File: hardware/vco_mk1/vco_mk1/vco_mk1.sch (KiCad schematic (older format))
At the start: 86 parts, among them J1 power supply, J2 control in, J3 signal out, J4 Conn_01x03_Male, J5 BCM847 breakout socket, J6 Conn_01x01_Male, Q1 BCM847, Q2 BC547, Q3 BC547, Q4 2N7000, Q5 BC547, Q6 BC327, U1 LM324, U2 LM324, U3 74HC86

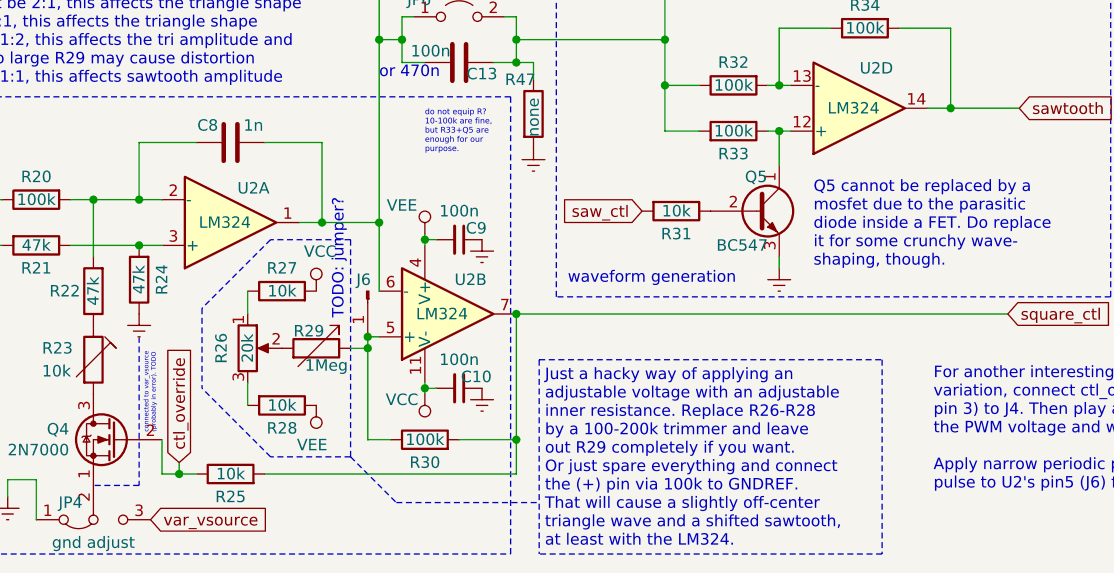
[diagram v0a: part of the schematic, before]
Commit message: triangle center adjust: add 0-Ohm-resistor to GNDREF
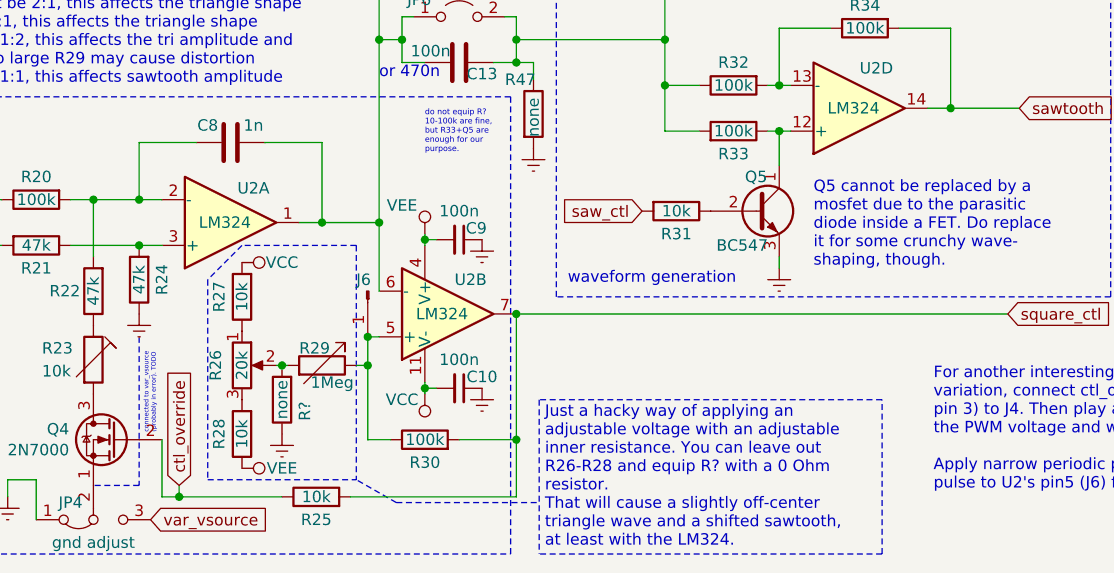
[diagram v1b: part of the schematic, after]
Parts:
- added R?: none, Resistor_SMD:R_0805_2012Metric_Pad1.15x1.40mm_HandSolder, symbol Device:R
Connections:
- net GNDREF: now also R?.1
- net at R26.2, R29.2: now also R?.2
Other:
- note added: "Just a hacky way of applying an\nadjustable voltage with an adjustable\ninner resistance. You can leave out\nR26-R28 and equip R? with a 0 Ohm\nresistor.\nThat will cause a slightly off-center\ntriangle wave and a shifted sawtooth,\nat least with the LM324."
- note removed: "Just a hacky way of applying an\nadjustable voltage with an adjustable\ninner resistance. Replace R26-R28\nby a 100-200k trimmer and leave\nout R29 completely if you want.\nOr just spare everything and connect\nthe (+) pin via 100k to GNDREF.\nThat will cause a slightly off-center\ntriangle wave and a shifted sawtooth,\nat least with the LM324."
- note removed: "TODO: jumper?"
- moved on the sheet: R25, R26, R27, R28, R29
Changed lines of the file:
@@
 $EndComp
 Wire Wire Line
-	2375 7400 3475 7400
-Wire Wire Line
-	3475 7400 3475 7250
+	2750 7500 3475 7500
+Wire Wire Line
+	3475 7500 3475 7250
 Wire Wire Line
 	3475 7250 3475 6700
@@
 Wire Wire Line
 	2875 6800 2825 6800
-Wire Wire Line
-	2825 6800 2825 6850
 $Comp
 L power:VCC #PWR026
@@
 U 1 1 5D5CE3BE
 P 3225 7025
-F 0 "C10" V 3175 7100 50  0000 C CNN
+F 0 "C10" V 3175 7125 50  0000 C CNN
 F 1 "100n" V 3100 7025 50  0000 C CNN
 F 2 "Capacitor_SMD:C_0805_2012Metric_Pad1.15x1.40mm_HandSolder" H 3225 7025 50  0001 C CNN
@@
 L Device:R R27
 U 1 1 5D9107CB
-P 2450 6600
-F 0 "R27" V 2550 6600 50  0000 C CNN
-F 1 "10k" V 2450 6600 50  0000 C CNN
-F 2 "Resistor_SMD:R_0805_2012Metric_Pad1.15x1.40mm_HandSolder" V 2380 6600 50  0001 C CNN
-F 3 "~" H 2450 6600 50  0001 C CNN
-	1    2450 6600
-	0    -1   -1   0
+P 2275 6625
+F 0 "R27" V 2375 6625 50  0000 C CNN
+F 1 "10k" V 2275 6625 50  0000 C CNN
+F 2 "Resistor_SMD:R_0805_2012Metric_Pad1.15x1.40mm_HandSolder" V 2205 6625 50  0001 C CNN
+F 3 "~" H 2275 6625 50  0001 C CNN
+	1    2275 6625
+	-1   0    0    1
 $EndComp
 $Comp
 L Device:R R28
 U 1 1 5D910D8F
-P 2450 7100
-F 0 "R28" V 2550 7100 50  0000 C CNN
-F 1 "10k" V 2450 7100 50  0000 C CNN
-F 2 "Resistor_SMD:R_0805_2012Metric_Pad1.15x1.40mm_HandSolder" V 2380 7100 50  0001 C CNN
-F 3 "~" H 2450 7100 50  0001 C CNN
-	1    2450 7100
-	0    1    1    0
+P 2275 7225
+F 0 "R28" V 2375 7225 50  0000 C CNN
+F 1 "10k" V 2275 7225 50  0000 C CNN
+F 2 "Resistor_SMD:R_0805_2012Metric_Pad1.15x1.40mm_HandSolder" V 2205 7225 50  0001 C CNN
+F 3 "~" H 2275 7225 50  0001 C CNN
+	1    2275 7225
+	-1   0    0    1
 $EndComp
 $Comp
 L Device:R_POT R26
 U 1 1 5D911866
-P 2300 6850
-F 0 "R26" V 2185 6850 50  0000 C CNN
-F 1 "20k" V 2300 6850 50  0000 C CNN
-F 2 "Potentiometer_THT:Potentiometer_Runtron_RM-065_Vertical" H 2300 6850 50  0001 C CNN
-F 3 "~" H 2300 6850 50  0001 C CNN
-	1    2300 6850
+P 2275 6925
+F 0 "R26" V 2160 6925 50  0000 C CNN
+F 1 "20k" V 2275 6925 50  0000 C CNN
+F 2 "Potentiometer_THT:Potentiometer_Runtron_RM-065_Vertical" H 2275 6925 50  0001 C CNN
+F 3 "~" H 2275 6925 50  0001 C CNN
+	1    2275 6925
 	1    0    0    -1
 $EndComp
@@
 L power:VEE #PWR024
 U 1 1 5D92BF20
-P 2600 7100
-F 0 "#PWR024" H 2600 6950 50  0001 C CNN
-F 1 "VEE" H 2618 7273 50  0000 C CNN
-F 2 "" H 2600 7100 50  0001 C CNN
-F 3 "" H 2600 7100 50  0001 C CNN
-	1    2600 7100
-	-1   0    0    1
+P 2275 7375
+F 0 "#PWR024" H 2275 7225 50  0001 C CNN
+F 1 "VEE" V 2275 7550 50  0000 C CNN
+F 2 "" H 2275 7375 50  0001 C CNN
+F 3 "" H 2275 7375 50  0001 C CNN
+	1    2275 7375
+	0    1    1    0
 $EndComp
 $Comp
 L power:VCC #PWR023
 U 1 1 5D931D60
-P 2600 6600
-F 0 "#PWR023" H 2600 6450 50  0001 C CNN
-F 1 "VCC" H 2617 6773 50  0000 C CNN
-F 2 "" H 2600 6600 50  0001 C CNN
-F 3 "" H 2600 6600 50  0001 C CNN
-	1    2600 6600
-	1    0    0    -1
+P 2275 6475
+F 0 "#PWR023" H 2275 6325 50  0001 C CNN
+F 1 "VCC" V 2275 6650 50  0000 C CNN
+F 2 "" H 2275 6475 50  0001 C CNN
+F 3 "" H 2275 6475 50  0001 C CNN
+	1    2275 6475
+	0    1    1    0
 $EndComp
 $Comp
 L Device:R_Variable R29
 U 1 1 5D95EF15
-P 2600 6850
-F 0 "R29" V 2675 6750 50  0000 L CNN
-F 1 "1Meg" V 2525 6800 50  0000 L CNN
-F 2 "Potentiometer_THT:Potentiometer_Runtron_RM-065_Vertical" V 2530 6850 50  0001 C CNN
-F 3 "~" H 2600 6850 50  0001 C CNN
-	1    2600 6850
+P 2625 6925
+F 0 "R29" V 2700 6825 50  0000 L CNN
+F 1 "1Meg" V 2550 6875 50  0000 L CNN
+F 2 "Potentiometer_THT:Potentiometer_Runtron_RM-065_Vertical" V 2555 6925 50  0001 C CNN
+F 3 "~" H 2625 6925 50  0001 C CNN
+	1    2625 6925
 	0    1    -1   0
 $EndComp
@@
 $EndComp
 Wire Wire Line
-	2000 7400 2075 7400
-Wire Wire Line
-	2000 7350 2000 7400
-Text GLabel 2000 7350 1    50   Input ~ 0
+	2000 7500 2450 7500
+Wire Wire Line
+	2000 7450 2000 7500
+Text GLabel 2000 7450 1    50   Input ~ 0
 ctl_override
-Connection ~ 2000 7400
-Wire Wire Line
-	1925 7400 2000 7400
-Wire Wire Line
-	1925 7250 1925 7400
 $Comp
 L Transistor_FET:2N7000 Q4
@@
 L Device:R R25
 U 1 1 5CF3A8E6
-P 2225 7400
-F 0 "R25" V 2125 7400 50  0000 C CNN
-F 1 "10k" V 2225 7400 50  0000 C CNN
-F 2 "Resistor_SMD:R_0805_2012Metric_Pad1.15x1.40mm_HandSolder" V 2155 7400 50  0001 C CNN
-F 3 "~" H 2225 7400 50  0001 C CNN
-	1    2225 7400
+P 2600 7500
+F 0 "R25" V 2500 7500 50  0000 C CNN
+F 1 "10k" V 2600 7500 50  0000 C CNN
+F 2 "Resistor_SMD:R_0805_2012Metric_Pad1.15x1.40mm_HandSolder" V 2530 7500 50  0001 C CNN
+F 3 "~" H 2600 7500 50  0001 C CNN
+	1    2600 7500
 	0    -1   -1   0
 $EndComp
@@
 	1    0    0    -1
 $EndComp
-Wire Wire Line
-	2300 6600 2300 6700
-Wire Wire Line
-	2300 7100 2300 7000
-Wire Wire Line
-	2750 6850 2825 6850
-Connection ~ 2825 6850
-Wire Wire Line
-	2825 6850 2825 7250
-Wire Notes Line
-	2750 6375 2400 6375
-Wire Notes Line
-	2750 7325 2400 7325
-Wire Notes Line
-	2750 6375 2750 7325
-Wire Notes Line
-	2400 7325 2100 7025
-Wire Notes Line
-	2400 6375 2100 6675
-Wire Notes Line
-	2100 6675 2100 7025
-Wire Notes Line
-	2750 7325 2950 7525
 Text Notes 3600 7725 0    50   ~ 0
-Just a hacky way of applying an\nadjustable voltage with an adjustable\ninner resistance. Replace R26-R28\nby a 100-200k trimmer and leave\nout R29 completely if you want.\nOr just spare everything and connect\nthe (+) pin via 100k to GNDREF.\nThat will cause a slightly off-center\ntriangle wave and a shifted sawtooth,\nat least with the LM324.
-Wire Notes Line
-	3575 6900 5075 6900
-Wire Notes Line
-	5075 6900 5075 7750
+Just a hacky way of applying an\nadjustable voltage with an adjustable\ninner resistance. You can leave out\nR26-R28 and equip R? with a 0 Ohm\nresistor.\nThat will cause a slightly off-center\ntriangle wave and a shifted sawtooth,\nat least with the LM324.
 Wire Notes Line
 	5075 7750 3575 7750
-Wire Notes Line
-	3575 6900 3575 7750
 $Comp
 L power:GNDREF #PWR029
@@
 	3975 2125 3975 3200
 Connection ~ 3800 3200
-Text Notes 2725 6725 1    50   ~ 0
-TODO: jumper?
 $Comp
 L Connector:Conn_01x01_Male J6
@@
 	0    1    1    0
 $EndComp
+Wire Wire Line
+	1925 7500 2000 7500
+Wire Wire Line
+	1925 7250 1925 7500
+Connection ~ 2000 7500
+Wire Wire Line
+	2825 6800 2825 6925
+Wire Wire Line
+	2425 6925 2450 6925
+Wire Wire Line
+	2775 6925 2825 6925
+Connection ~ 2825 6925
+Wire Wire Line
+	2825 6925 2825 7250
+$Comp
+L Device:R R?
+U 1 1 5D5E77C1
+P 2450 7075
+F 0 "R?" V 2350 7125 50  0000 C CNN
+F 1 "none" V 2450 7075 50  0000 C CNN
+F 2 "Resistor_SMD:R_0805_2012Metric_Pad1.15x1.40mm_HandSolder" V 2380 7075 50  0001 C CNN
+F 3 "~" H 2450 7075 50  0001 C CNN
+	1    2450 7075
+	-1   0    0    1
+$EndComp
+Connection ~ 2450 6925
+Wire Wire Line
+	2450 6925 2475 6925
+$Comp
+L power:GNDREF #PWR?
+U 1 1 5D5E8B33
+P 2450 7225
+F 0 "#PWR?" H 2450 6975 50  0001 C CNN
+F 1 "GNDREF" H 2455 7052 50  0001 C CNN
+F 2 "" H 2450 7225 50  0001 C CNN
+F 3 "" H 2450 7225 50  0001 C CNN
+	1    2450 7225
+	1    0    0    -1
+$EndComp
+Wire Notes Line
+	2775 6400 2275 6400
+Wire Notes Line
+	2125 6550 2125 7425
+Wire Notes Line
+	2125 7425 2775 7425
+Wire Notes Line
+	2775 6400 2775 7425
+Wire Notes Line
+	2275 6400 2125 6550
+Wire Notes Line
+	2950 7525 2775 7425
+Wire Notes Line
+	5075 7750 5075 7075
+Wire Notes Line
+	5075 7075 3575 7075
+Wire Notes Line
+	3575 7075 3575 7750
 $EndSCHEMATC
